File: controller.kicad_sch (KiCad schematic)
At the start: 13 parts, among them J601 Prog, U601 STM32L151C8Tx

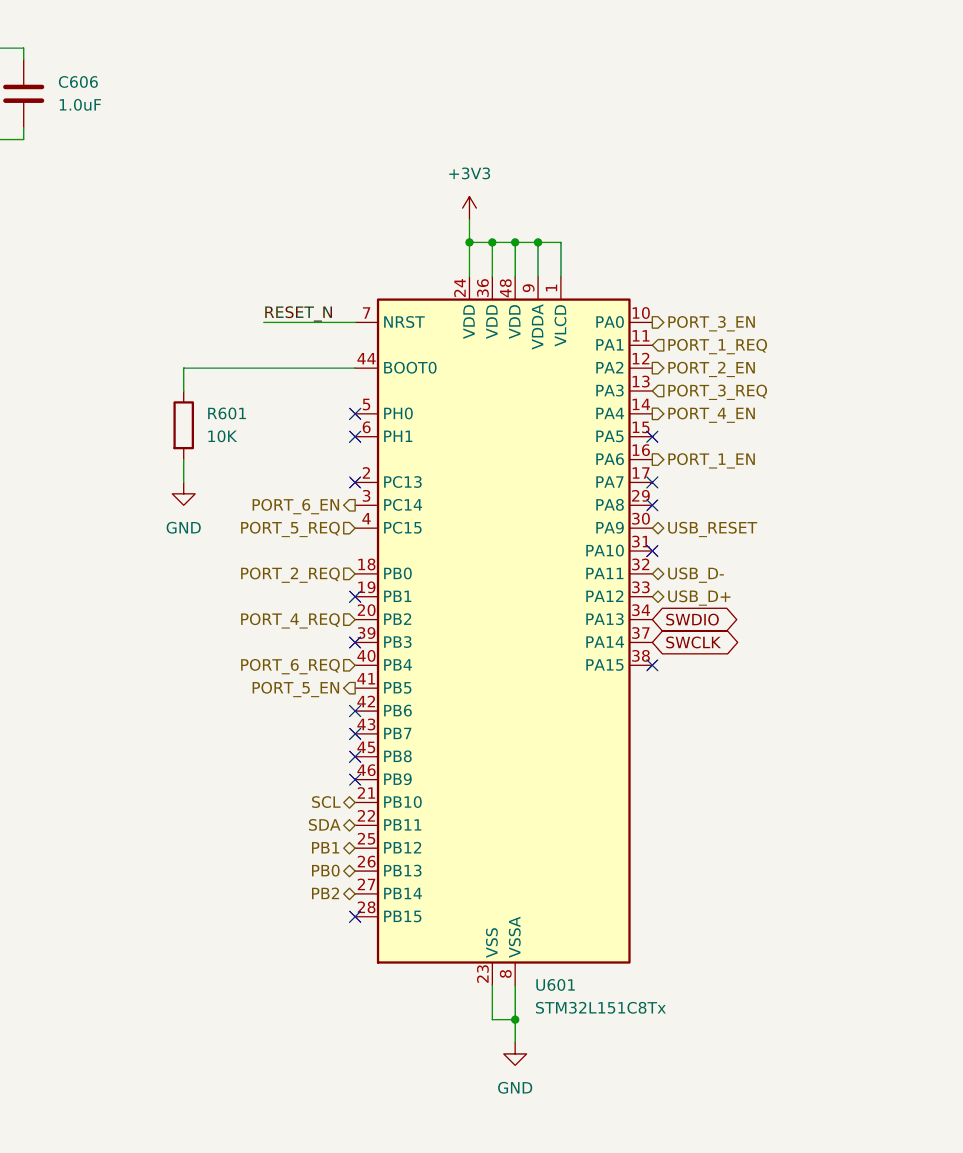
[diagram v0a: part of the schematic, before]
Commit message: Commit old worktree
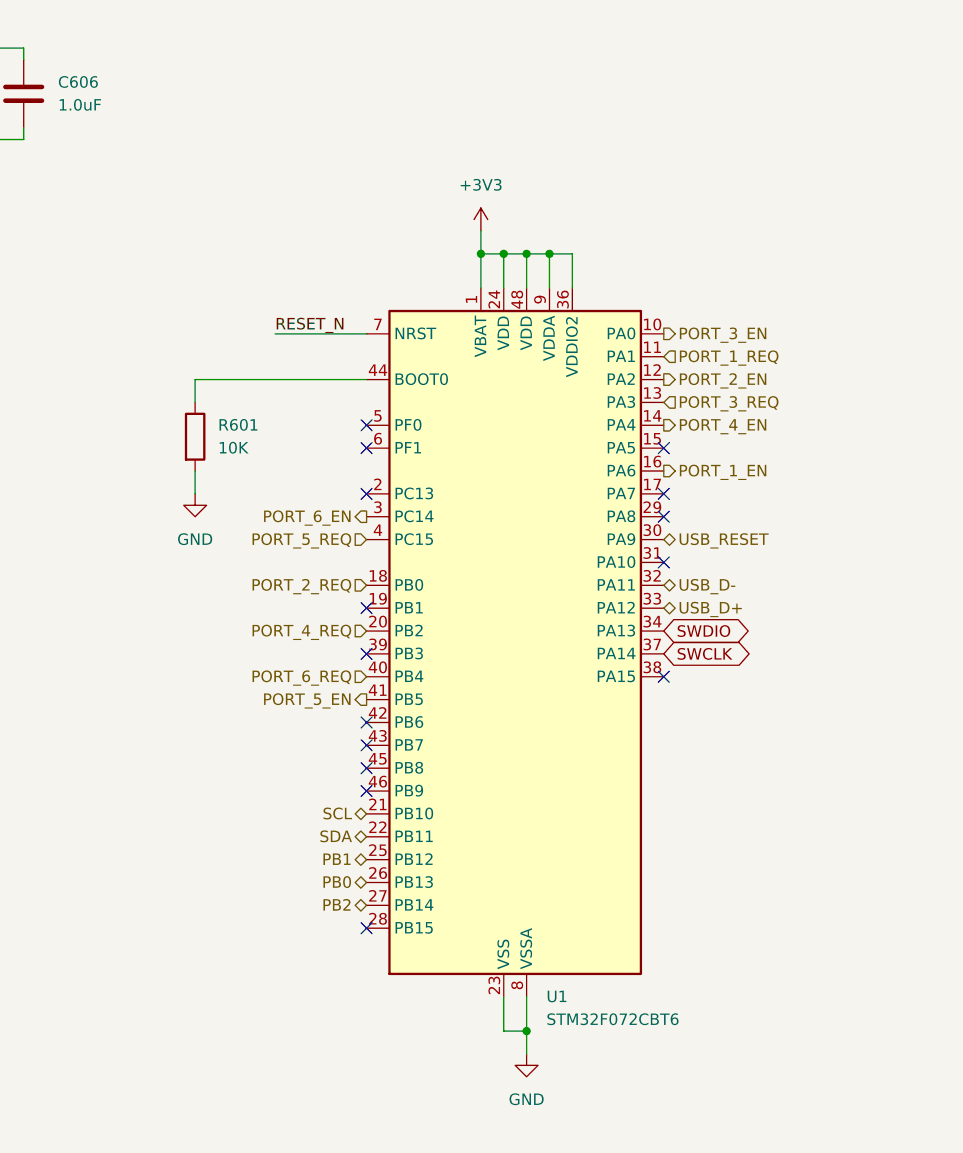
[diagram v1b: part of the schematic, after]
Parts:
- removed U601: STM32L151C8Tx, Package_QFP:LQFP-48_7x7mm_P0.5mm, symbol MCU_ST_STM32L1:STM32L151C8Tx
- added U1: STM32F072CBT6, Package_QFP:LQFP-48_7x7mm_P0.5mm, symbol MCU_ST_STM32F0:STM32F072CBTx
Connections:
- net +3V3: now also U1.1 (VBAT), U1.24 (VDD), U1.36 (VDDIO2), U1.48 (VDD), U1.9 (VDDA)
- net GND: now also U1.23 (VSS), U1.35 (VSS), U1.47 (VSS), U1.8 (VSSA)
- net PB0: now also U1.26 (PB13)
- net PB1: now also U1.25 (PB12)
- net PB2: now also U1.27 (PB14)
- net PORT_1_EN: now also U1.16 (PA6)
- net PORT_1_REQ: now also U1.11 (PA1)
- net PORT_2_EN: now also U1.12 (PA2)
- net PORT_2_REQ: now also U1.18 (PB0)
- net PORT_3_EN: now also U1.10 (PA0)
- net PORT_3_REQ: now also U1.13 (PA3)
- net PORT_4_EN: now also U1.14 (PA4)
- net PORT_4_REQ: now also U1.20 (PB2)
- net PORT_5_EN: now also U1.41 (PB5)
- net PORT_5_REQ: now also U1.4 (PC15)
- net PORT_6_EN: now also U1.3 (PC14)
- net PORT_6_REQ: now also U1.40 (PB4)
- net RESET_N: now also U1.7 (NRST)
- net SCL: now also U1.21 (PB10)
- net SDA: now also U1.22 (PB11)
- net SWCLK: now also U1.37 (PA14)
- net SWDIO: now also U1.34 (PA13)
- net USB_D+: now also U1.33 (PA12)
- net USB_D-: now also U1.32 (PA11)
- net USB_RESET: now also U1.30 (PA9)
- net at R601.1: now also U1.44 (BOOT0)
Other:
- moved on the sheet: R601
